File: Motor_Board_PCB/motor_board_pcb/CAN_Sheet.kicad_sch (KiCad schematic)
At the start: 14 parts, among them J1 CAN_OUT

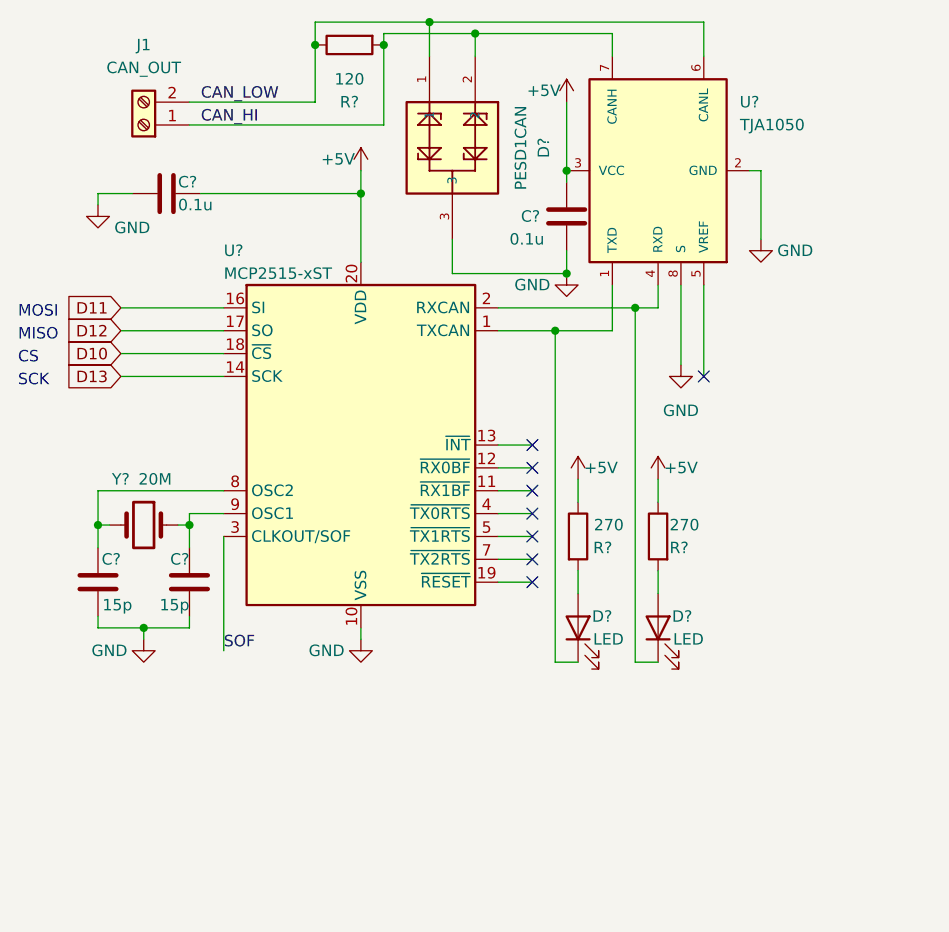
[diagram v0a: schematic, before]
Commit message: Schematic changes before sending to kim
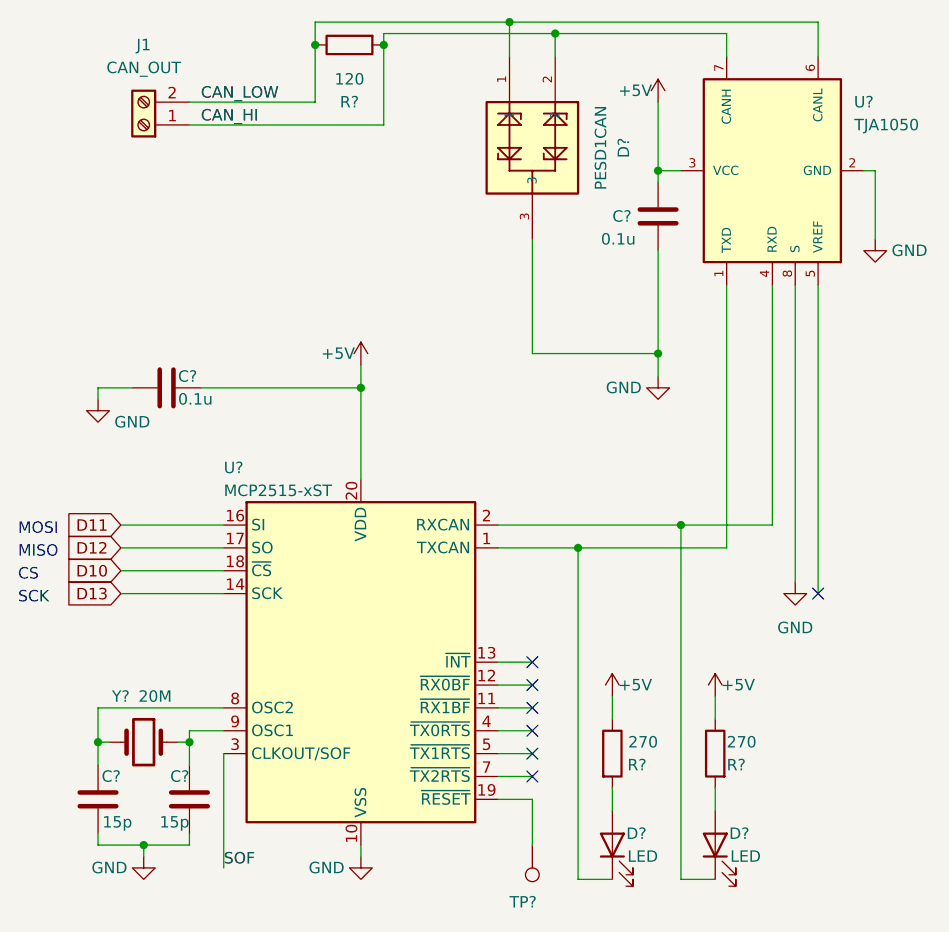
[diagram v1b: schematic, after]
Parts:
- added TP?: TestPoint, TestPoint:TestPoint_Pad_D1.0mm, symbol Connector:TestPoint
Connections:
- net at U?.19 (~{RESET}): now also TP?.1
- no-connect marks 8 -> 7
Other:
- moved on the sheet: C?, D?, R?, U?, Y?
